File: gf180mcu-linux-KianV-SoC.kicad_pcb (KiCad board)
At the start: 4 copper layers, 94.7 x 52 mm, 65 parts, among them CN1 HC-PBB40C-70DS-0.4V-2.0-02_CU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, J1 Micro_SD_Card, J2 Conn_01x06_Pin, J3 Conn_01x06_Pin, J4 Conn_02x06_Top_Bottom_custom, J5 USB_C_Receptacle_PowerOnly_6P, SW1 SW_Push, U1 MT48LC16M16A2P, U2 TPS3808DBV, U3 TLV62569DBV, Y1 CXO_DIP8

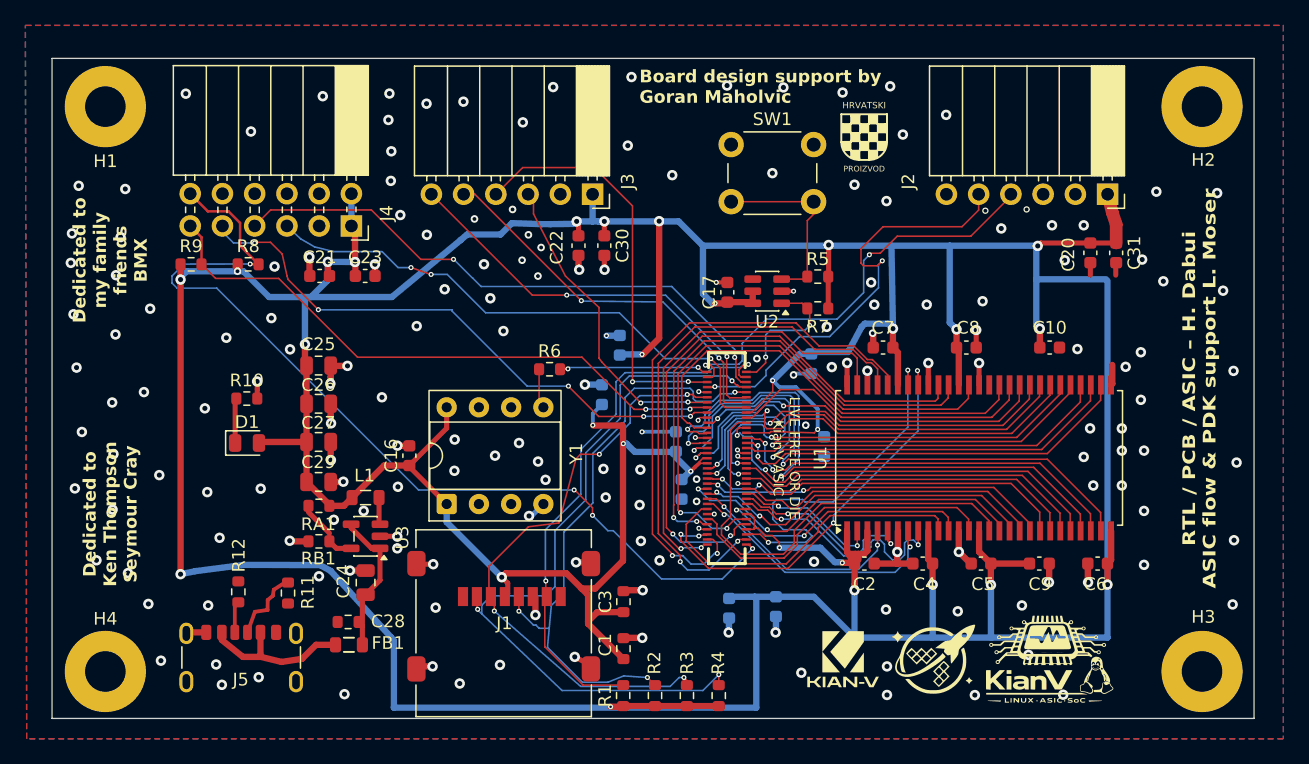
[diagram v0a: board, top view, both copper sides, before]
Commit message: small tweaks
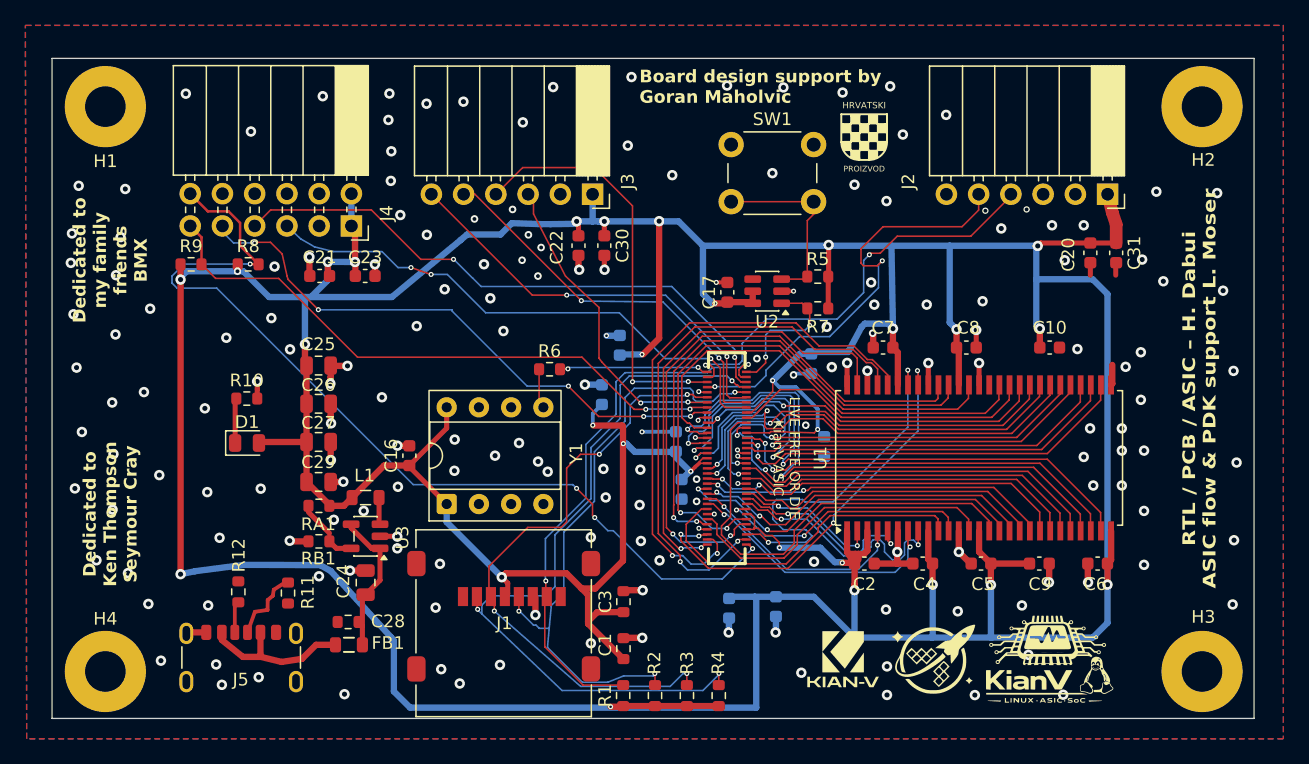
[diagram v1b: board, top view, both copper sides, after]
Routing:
- net GND: track 69.8 -> 63.4 mm, vias 187 -> 186
- net /3V3: track 487.0 -> 485.0 mm
- net /SPI0_MOSI: track 46.8 -> 48.2 mm
- net /SPI0_SCLK: track 47.0 -> 47.8 mm
